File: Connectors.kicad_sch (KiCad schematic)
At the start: 4 parts, among them J1 Conn_01x04_Pin, J2 Conn_01x04_Pin, J3 Conn_01x09_Pin, J4 Conn_02x03_Odd_Even

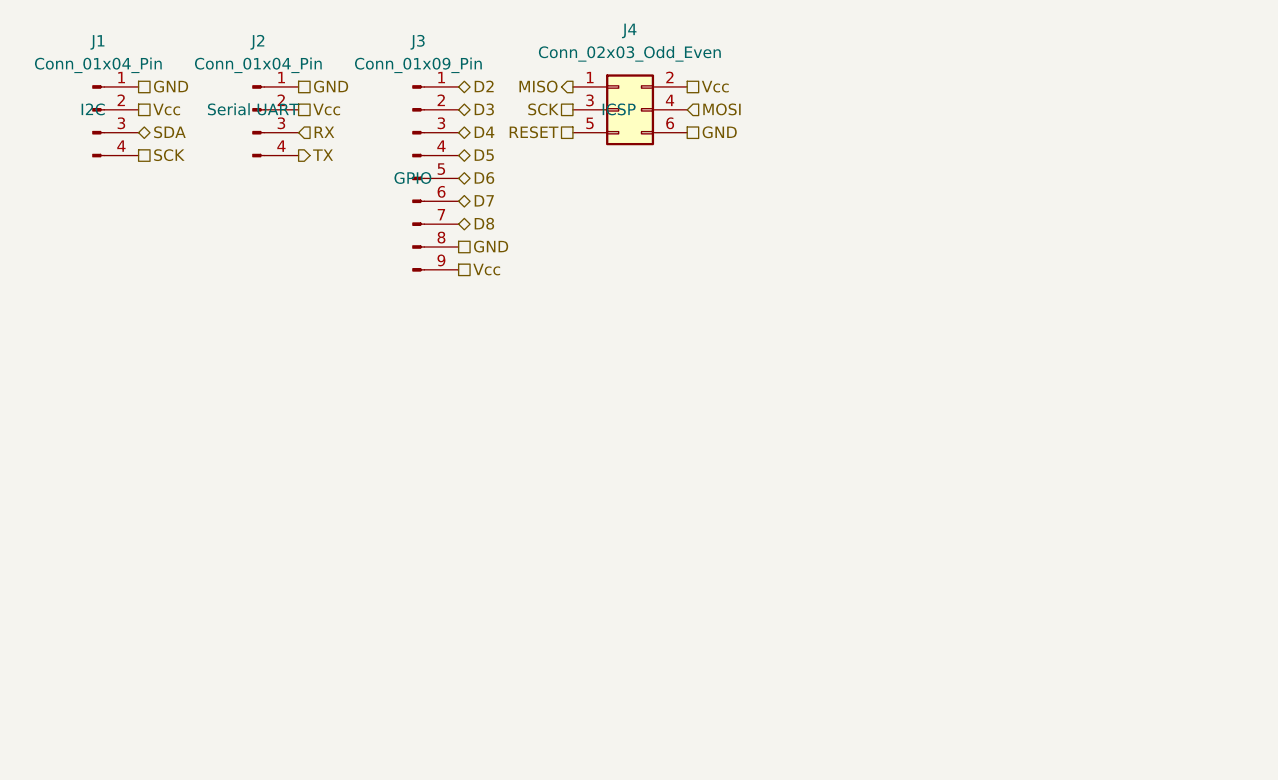
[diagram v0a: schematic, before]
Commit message: Completed comments.
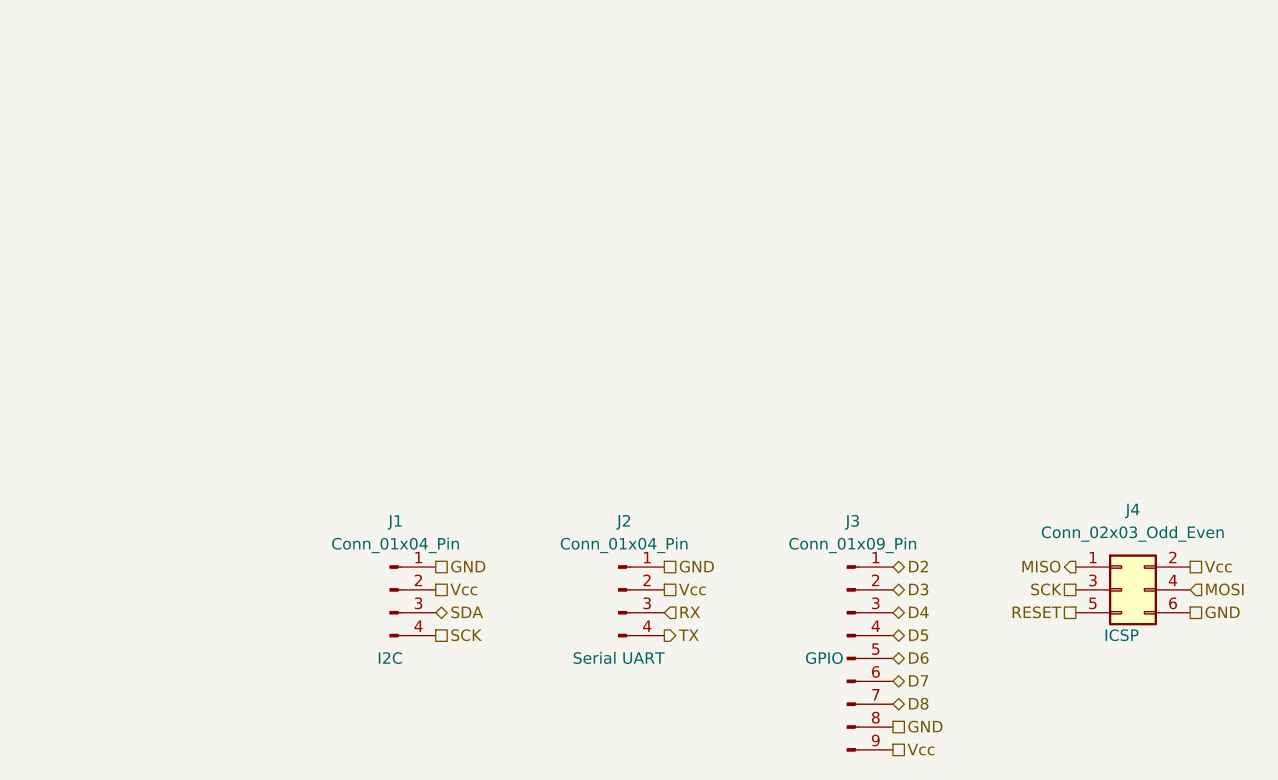
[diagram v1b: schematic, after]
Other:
- moved on the sheet: J1, J2, J3, J4
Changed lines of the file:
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@@
 	(hierarchical_label "RX"
 		(shape input)
-		(at 93.98 43.18 0)
+		(at 134.62 96.52 0)
 		(effects
 			(font
@@
 	(hierarchical_label "D7"
 		(shape bidirectional)
-		(at 111.76 50.8 0)
+		(at 160.02 104.14 0)
 		(effects
 			(font
@@
 	(hierarchical_label "D2"
 		(shape bidirectional)
-		(at 111.76 38.1 0)
+		(at 160.02 91.44 0)
 		(effects
 			(font
@@
 	(hierarchical_label "RESET"
 		(shape passive)
-		(at 124.46 43.18 180)
+		(at 180.34 96.52 180)
 		(effects
 			(font
@@
 	(hierarchical_label "Vcc"
 		(shape passive)
-		(at 93.98 40.64 0)
+		(at 134.62 93.98 0)
 		(effects
 			(font
@@
 	(hierarchical_label "Vcc"
 		(shape passive)
-		(at 137.16 38.1 0)
+		(at 193.04 91.44 0)
 		(effects
 			(font
@@
 	(hierarchical_label "MOSI"
 		(shape input)
-		(at 137.16 40.64 0)
+		(at 193.04 93.98 0)
 		(effects
 			(font
@@
 	(hierarchical_label "D5"
 		(shape bidirectional)
-		(at 111.76 45.72 0)
+		(at 160.02 99.06 0)
 		(effects
 			(font
@@
 	(hierarchical_label "GND"
 		(shape passive)
-		(at 93.98 38.1 0)
+		(at 134.62 91.44 0)
 		(effects
 			(font
@@
 	(hierarchical_label "TX"
 		(shape output)
-		(at 93.98 45.72 0)
+		(at 134.62 99.06 0)
 		(effects
 			(font
@@
 	(hierarchical_label "D4"
 		(shape bidirectional)
-		(at 111.76 43.18 0)
+		(at 160.02 96.52 0)
 		(effects
 			(font
@@
 	(hierarchical_label "MISO"
 		(shape output)
-		(at 124.46 38.1 180)
+		(at 180.34 91.44 180)
 		(effects
 			(font
@@
 	(hierarchical_label "Vcc"
 		(shape passive)
-		(at 76.2 40.64 0)
+		(at 109.22 93.98 0)
 		(effects
 			(font
@@
 	(hierarchical_label "D8"
 		(shape bidirectional)
-		(at 111.76 53.34 0)
+		(at 160.02 106.68 0)
 		(effects
 			(font
@@
 	(hierarchical_label "GND"
 		(shape passive)
-		(at 137.16 43.18 0)
+		(at 193.04 96.52 0)
 		(effects
 			(font
@@
 	(hierarchical_label "GND"
 		(shape passive)
-		(at 76.2 38.1 0)
+		(at 109.22 91.44 0)
 		(effects
 			(font
@@
 	(hierarchical_label "SCK"
 		(shape passive)
-		(at 124.46 40.64 180)
+		(at 180.34 93.98 180)
 		(effects
 			(font
@@
 	(hierarchical_label "SCK"
 		(shape passive)
-		(at 76.2 45.72 0)
+		(at 109.22 99.06 0)
 		(effects
 			(font
@@
 	(hierarchical_label "GND"
 		(shape passive)
-		(at 111.76 55.88 0)
+		(at 160.02 109.22 0)
 		(effects
 			(font
@@
 	(hierarchical_label "D6"
 		(shape bidirectional)
-		(at 111.76 48.26 0)
+		(at 160.02 101.6 0)
 		(effects
 			(font
@@
 	(hierarchical_label "Vcc"
 		(shape passive)
-		(at 111.76 58.42 0)
+		(at 160.02 111.76 0)
 		(effects
 			(font
@@
 	(hierarchical_label "SDA"
 		(shape bidirectional)
-		(at 76.2 43.18 0)
+		(at 109.22 96.52 0)
 		(effects
 			(font
@@
 	(hierarchical_label "D3"
 		(shape bidirectional)
-		(at 111.76 40.64 0)
+		(at 160.02 93.98 0)
 		(effects
 			(font
@@
 	(symbol
 		(lib_id "Connector:Conn_01x09_Pin")
-		(at 106.68 48.26 0)
+		(at 154.94 101.6 0)
 		(unit 1)
 		(exclude_from_sim no)
@@
 		(on_board yes)
 		(dnp no)
-		(fields_autoplaced yes)
 		(property "Reference" "J3"
-			(at 107.315 33.02 0)
+			(at 155.575 86.36 0)
 			(effects
 				(font
@@
 		)
 		(property "Value" "Conn_01x09_Pin"
-			(at 107.315 35.56 0)
+			(at 155.575 88.9 0)
 			(effects
 				(font
@@
 		)
 		(property "Footprint" "Connector_PinHeader_2.54mm:PinHeader_1x09_P2.54mm_Vertical"
-			(at 106.68 48.26 0)
+			(at 154.94 101.6 0)
 			(effects
 				(font
@@
 		)
 		(property "Datasheet" "~"
-			(at 106.68 48.26 0)
+			(at 154.94 101.6 0)
 			(effects
 				(font
@@
 		)
 		(property "Description" "Generic connector, single row, 01x09, script generated"
-			(at 106.68 48.26 0)
+			(at 154.94 101.6 0)
 			(effects
 				(font
@@
 		)
 		(property "Purpose" "GPIO"
-			(at 106.68 48.26 0)
+			(at 152.4 101.6 0)
 			(effects
 				(font
@@
 	(symbol
 		(lib_id "Connector:Conn_01x04_Pin")
-		(at 71.12 40.64 0)
+		(at 104.14 93.98 0)
 		(unit 1)
 		(exclude_from_sim no)
@@
 		(on_board yes)
 		(dnp no)
-		(fields_autoplaced yes)
 		(property "Reference" "J1"
-			(at 71.755 33.02 0)
+			(at 104.775 86.36 0)
 			(effects
 				(font
@@
 		)
 		(property "Value" "Conn_01x04_Pin"
-			(at 71.755 35.56 0)
+			(at 104.775 88.9 0)
 			(effects
 				(font
@@
 		)
 		(property "Footprint" "Connector_PinHeader_2.54mm:PinHeader_1x04_P2.54mm_Vertical"
-			(at 71.12 40.64 0)
+			(at 104.14 93.98 0)
 			(effects
 				(font
@@
 		)
 		(property "Datasheet" "~"
-			(at 71.12 40.64 0)
+			(at 104.14 93.98 0)
 			(effects
 				(font
@@
 		)
 		(property "Description" "Generic connector, single row, 01x04, script generated"
-			(at 71.12 40.64 0)
+			(at 104.14 93.98 0)
 			(effects
 				(font
@@
 		)
 		(property "Purpose" "I2C"
-			(at 71.12 40.64 0)
+			(at 104.14 101.6 0)
 			(effects
 				(font
@@
 	(symbol
 		(lib_id "Connector:Conn_01x04_Pin")
-		(at 88.9 40.64 0)
+		(at 129.54 93.98 0)
 		(unit 1)
 		(exclude_from_sim no)
@@
 		(on_board yes)
 		(dnp no)
-		(fields_autoplaced yes)
 		(property "Reference" "J2"
-			(at 89.535 33.02 0)
+			(at 130.175 86.36 0)
 			(effects
 				(font
@@
 		)
 		(property "Value" "Conn_01x04_Pin"
-			(at 89.535 35.56 0)
+			(at 130.175 88.9 0)
 			(effects
 				(font
@@
 		)
 		(property "Footprint" "Connector_PinHeader_2.54mm:PinHeader_1x04_P2.54mm_Vertical"
-			(at 88.9 40.64 0)
+			(at 129.54 93.98 0)
 			(effects
 				(font
@@
 		)
 		(property "Datasheet" "~"
-			(at 88.9 40.64 0)
+			(at 129.54 93.98 0)
 			(effects
 				(font
@@
 		)
 		(property "Description" "Generic connector, single row, 01x04, script generated"
-			(at 88.9 40.64 0)
+			(at 129.54 93.98 0)
 			(effects
 				(font
@@
 		)
 		(property "Purpose" "Serial UART"
-			(at 88.9 40.64 0)
+			(at 129.54 101.6 0)
 			(effects
 				(font
@@
 	(symbol
 		(lib_id "Connector_Generic:Conn_02x03_Odd_Even")
-		(at 129.54 40.64 0)
+		(at 185.42 93.98 0)
 		(unit 1)
 		(exclude_from_sim no)
@@
 		(dnp no)
 		(property "Reference" "J4"
-			(at 130.81 31.75 0)
+			(at 186.69 85.09 0)
 			(effects
 				(font
@@
 		)
 		(property "Value" "Conn_02x03_Odd_Even"
-			(at 130.81 34.29 0)
+			(at 186.69 87.63 0)
 			(effects
 				(font
@@
 		)
 		(property "Footprint" "Connector_PinHeader_2.54mm:PinHeader_2x03_P2.54mm_Vertical"
-			(at 129.54 40.64 0)
+			(at 185.42 93.98 0)
 			(effects
 				(font
@@
 		)
 		(property "Datasheet" "~"
-			(at 129.54 40.64 0)
+			(at 185.42 93.98 0)
 			(effects
 				(font
@@
 		)
 		(property "Description" "Generic connector, double row, 02x03, odd/even pin numbering scheme (row 1 odd numbers, row 2 even numbers), script generated (kicad-library-utils/schlib/autogen/connector/)"
-			(at 129.54 40.64 0)
+			(at 185.42 93.98 0)
 			(effects
 				(font
@@
 		)
 		(property "Purpose" "ICSP"
-			(at 129.54 40.64 0)
-			(effects
-				(font
+			(at 185.42 99.06 0)
+			(effects
+				(font
